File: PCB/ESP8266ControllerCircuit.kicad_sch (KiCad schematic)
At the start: 14 parts, among them IC1 SN75176BDR, J1 Transmit, J2 Transmit, U1 JL850B-85003GA1, U2 EL3H7(B)(TA)-G, U3 JL850B-85003GA1, U4 DBT10-7.62-2P-GN

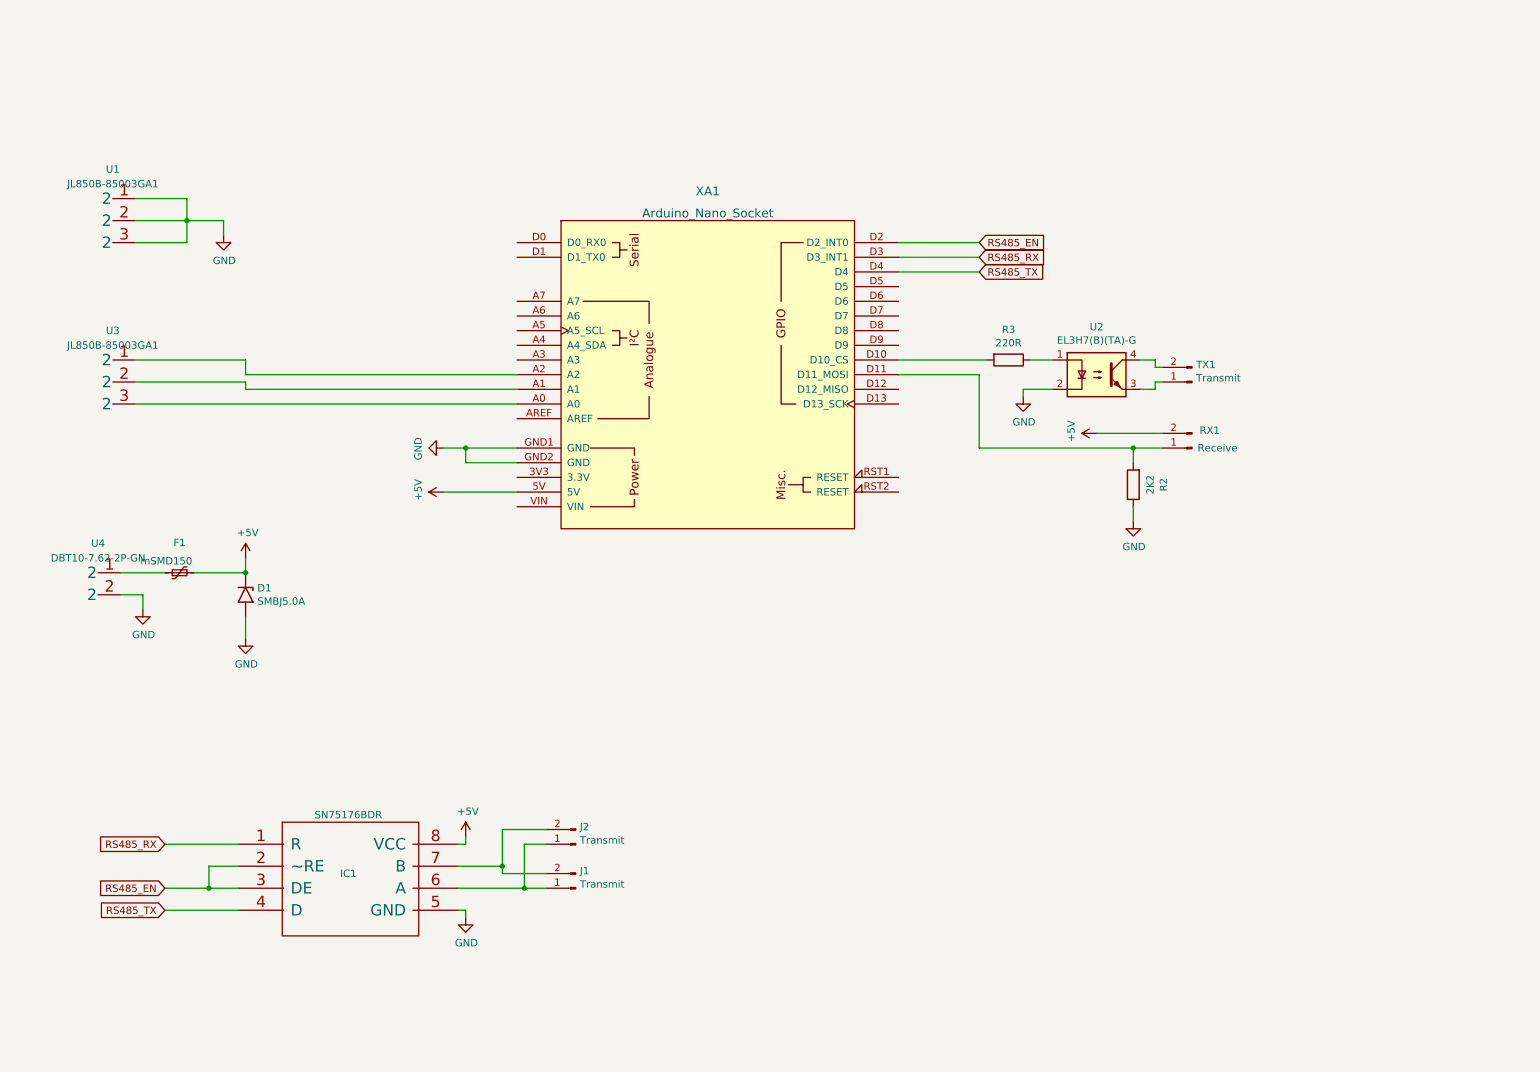
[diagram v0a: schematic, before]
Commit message: add
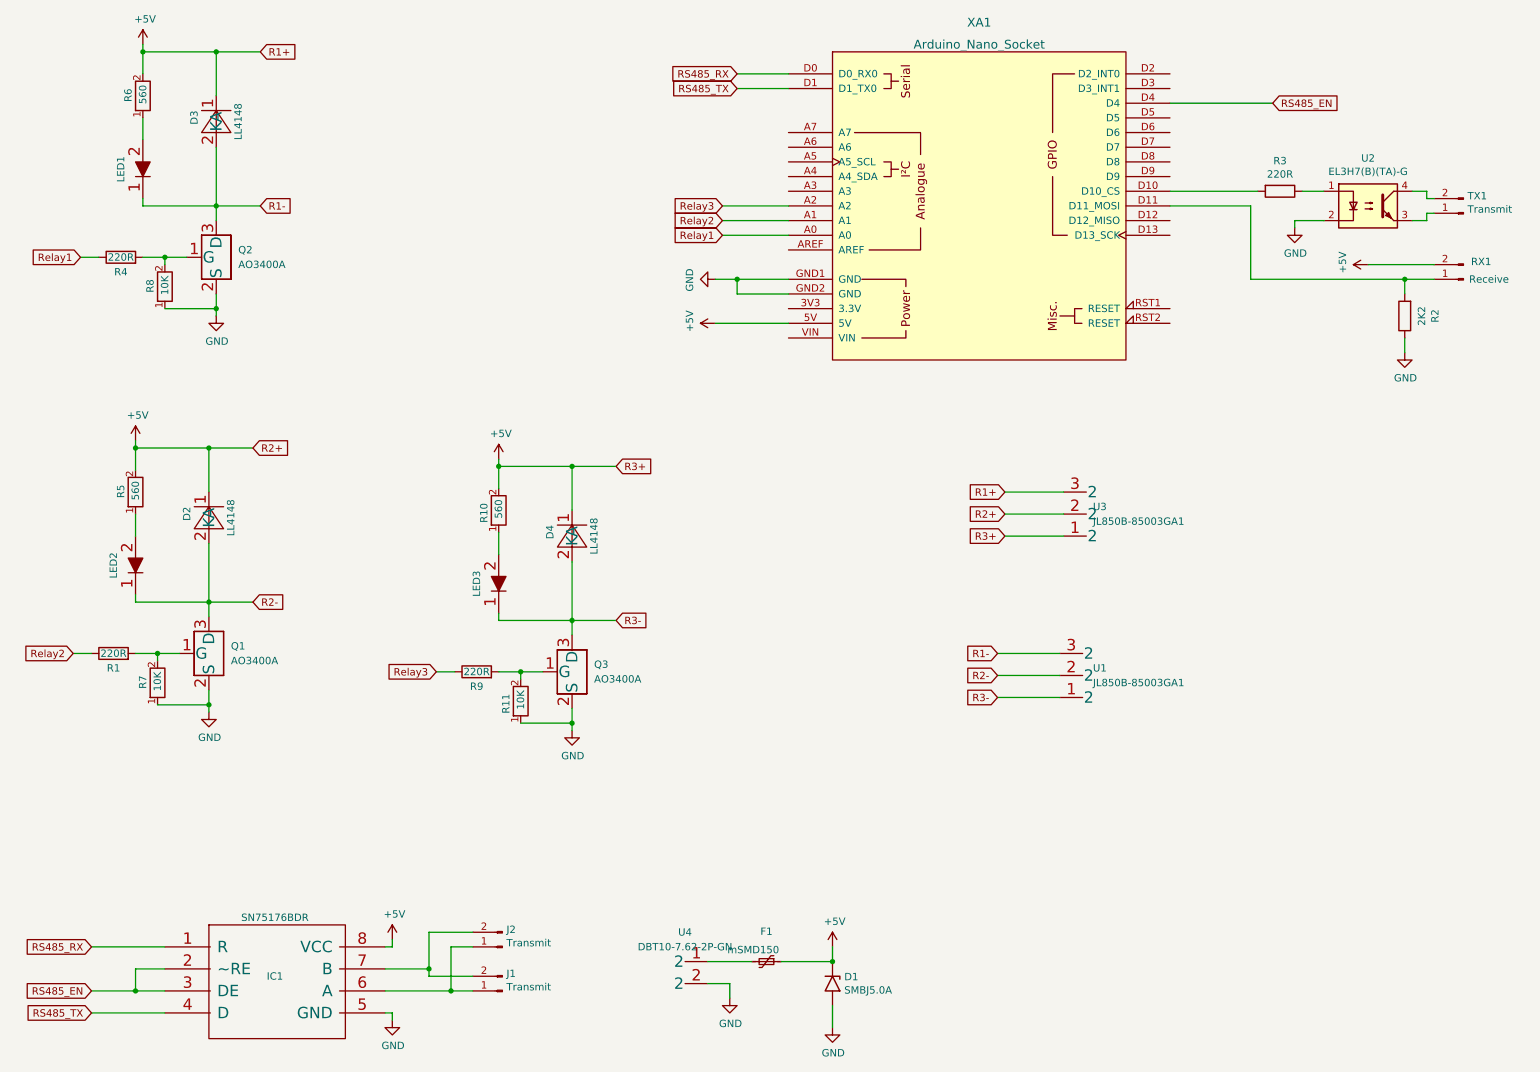
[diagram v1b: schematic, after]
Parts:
- added D2, D3, D4: LL4148, librarie2:LL4148, symbol librarie2:LL4148
- added LED1, LED2, LED3: 19-213_Y2C-CQ2R2L_3T_CY_, librarie2:19-213_Y2C-CQ2R2L_3T(CY), symbol librarie2:19-213_Y2C-CQ2R2L_3T_CY_
- added Q1, Q2, Q3: AO3400A, librarie2:AO3400A, symbol librarie2:AO3400A
- added R1, R4, R9: 220R, ModuleV440:resistor, symbol Device:R
- added R10, R5, R6: 560, ModuleV440:resistor, symbol librarie2:0805W8F5600T5E
- added R11, R7, R8: 10K, ModuleV440:resistor, symbol librarie2:0805W8F1002T5E
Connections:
- net +5V: now also U3.1 (2), U3.2, U3.3 (2), D2.1 (A), D3.1 (A), D4.1 (A), R10.2, R5.2, R6.2
- net GND: now also Q1.2 (S), Q2.2 (S), Q3.2 (S), R11.1, R7.1, R8.1; no longer U1.1 (2), U1.2, U1.3 (2)
- net RS485_EN: now also XA1.D4; no longer XA1.D2 (D2_INT0)
- net RS485_RX: now also XA1.D0 (D0_RX0); no longer XA1.D3 (D3_INT1)
- net RS485_TX: now also XA1.D1 (D1_TX0); no longer XA1.D4
- net Relay3: now reaches XA1.A2
- net Relay3: now also R9.1; no longer U3.1 (2)
- net Relay2: now reaches XA1.A1
- net Relay2: now also R1.1; no longer U3.2
- net Relay1: now reaches XA1.A0
- net Relay1: now also R4.1; no longer U3.3 (2)
- new net: LED2.2, R5.1
- new net: LED1.2, R6.1
- new net: Q2.1 (G), R4.2, R8.2
- new net: Q1.1 (G), R1.2, R7.2
- new net: LED3.2, R10.1
- new net: Q3.1 (G), R11.2, R9.2
- new net R1-: D3.2 (K), LED1.1, Q2.3 (D), U1.3 (2)
- new net R2-: D2.2 (K), LED2.1, Q1.3 (D), U1.2
- new net R3-: D4.2 (K), LED3.1, Q3.3 (D), U1.1 (2)
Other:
- moved on the sheet: D1, F1, IC1, J1, J2, R2, R3, RX1, TX1, U1, U2, U3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
